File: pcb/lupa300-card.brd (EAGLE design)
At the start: 45.7 x 65.7 mm, 39 parts

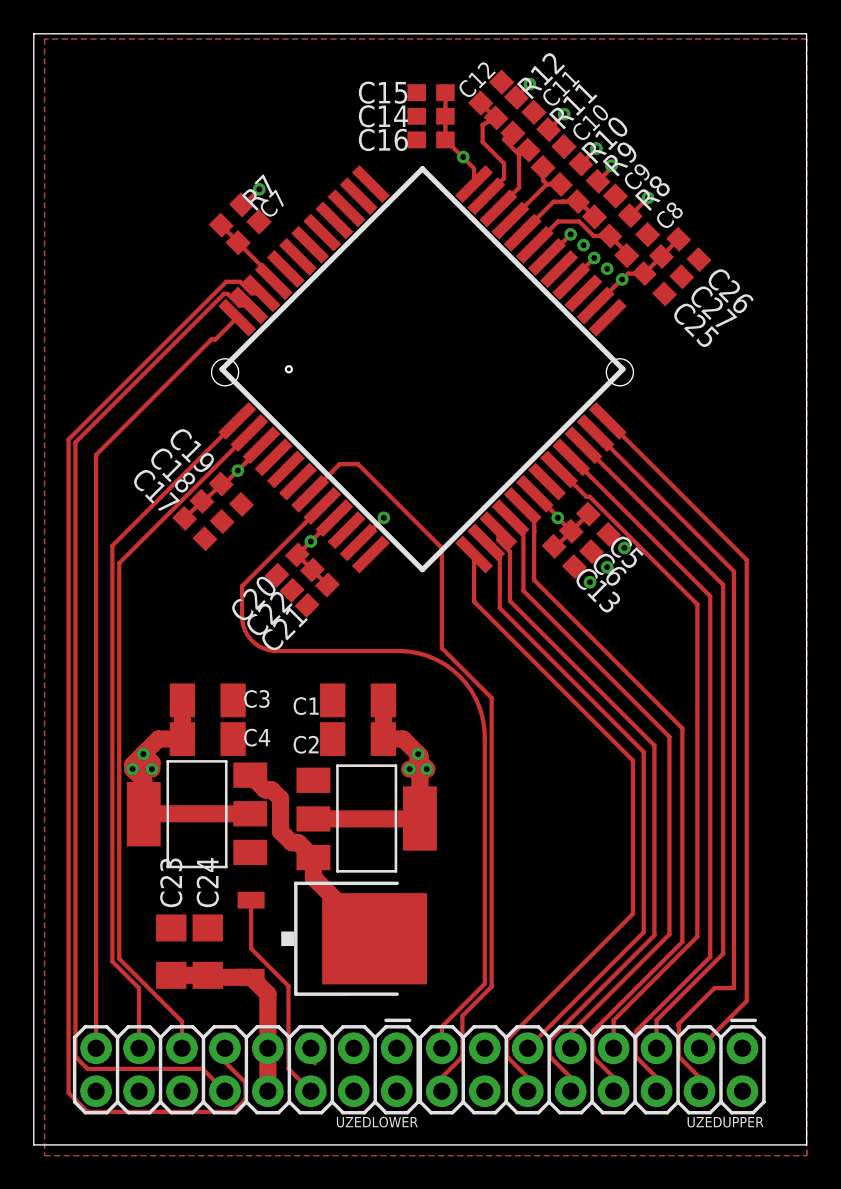
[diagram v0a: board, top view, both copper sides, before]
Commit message: routed critical signals.
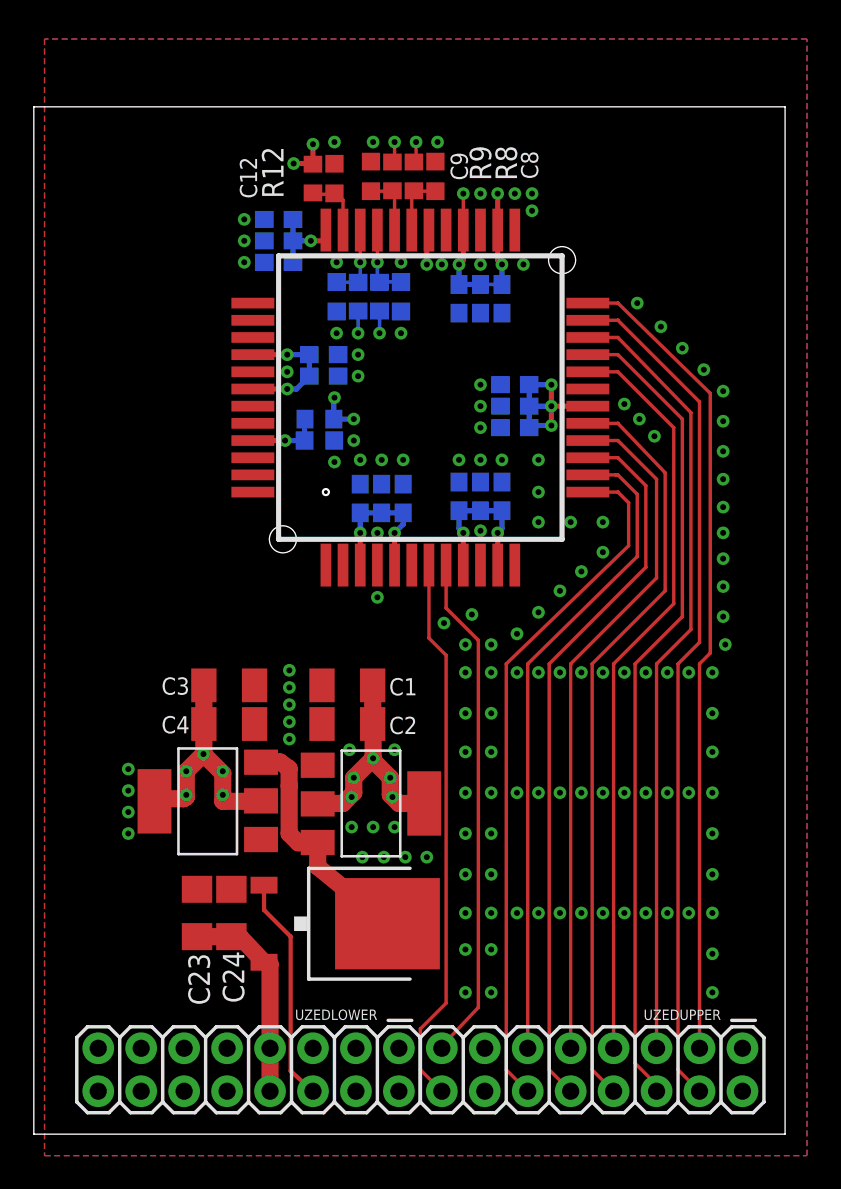
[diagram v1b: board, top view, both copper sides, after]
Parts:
- added C28, C29: (no value), rcl:C0603
- moved C11 15.1 mm to (17.9, 50.2), flipped to the bottom, turned to 270 degrees
- moved R11 14.1 mm to (19.2, 50.2), flipped to the bottom, turned to 90 degrees
- moved C9 14.0 mm to (19.9, 57.3), turned to 90 degrees
- moved R10 13.4 mm to (20.4, 50.2), flipped to the bottom, turned to 90 degrees
- moved R7 13.1 mm to (16.9, 42.9), flipped to the bottom, turned to 0 degrees
- moved C7 13.0 mm to (16.9, 41.7), flipped to the bottom, turned to 180 degrees
- moved C8 12.6 mm to (23.7, 57.3), turned to 90 degrees
- moved C15 12.6 mm to (14.5, 53.5), flipped to the bottom, turned to 0 degrees
- moved R8 12.5 mm to (22.5, 57.3), turned to 270 degrees
- moved C14 12.5 mm to (14.5, 52.2), flipped to the bottom, turned to 0 degrees
- moved C17 12.4 mm to (21.8, 38.2), flipped to the bottom, turned to 90 degrees
- moved C21 12.4 mm to (27.7, 38.4), flipped to the bottom, turned to 90 degrees
- moved C10 12.2 mm to (21.7, 50.2), flipped to the bottom, turned to 270 degrees
- moved R12 12.2 mm to (16.5, 57.1), turned to 270 degrees
- moved C22 11.6 mm to (26.4, 38.4), flipped to the bottom, turned to 90 degrees
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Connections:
- net 3V3: now also C28.1, C29.1
- net GND: now also C28.2, C29.2
- net SPI_CLK: now also UZEDLOWER.14; no longer UZEDLOWER.3
- net SPI_DATA: now also UZEDLOWER.16; no longer UZEDLOWER.5
- net SPI_EN: now also UZEDLOWER.12; no longer UZEDLOWER.1
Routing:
- net LINE_VALID: track 69.0 -> 0.00 mm
- net FRAME_VALID: track 60.2 -> 0.00 mm
- net INT_TIME3: track 46.8 -> 0.00 mm
- net INT_TIME1: track 41.1 -> 0.00 mm
- net INT_TIME2: track 40.8 -> 0.00 mm
- net CLK: track 45.3 -> 30.2 mm
- net 2.5V: track 60.9 -> 74.4 mm, vias 17 -> 26
- net RESET: track 45.1 -> 32.7 mm
- net D9: track 41.7 -> 48.4 mm
- net D7: track 40.7 -> 46.4 mm
- net D8: track 44.9 -> 50.4 mm
- net D6: track 43.2 -> 48.6 mm
- net 3V3: track 17.0 -> 22.3 mm, vias 3 -> 7
- net D5: track 39.8 -> 44.6 mm
- net BIAS1: track 7.93 -> 4.30 mm
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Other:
- board size 45.7 x 65.7 mm -> 44.4 x 60.8 mm
